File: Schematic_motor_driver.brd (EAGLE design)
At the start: 50 x 50 mm, 29 parts, among them Q2 IRF540, Q3 IRF540, Q4 IRF540, Q5 IRF540, U1 IR2104PBF, U2 IR2104PBF

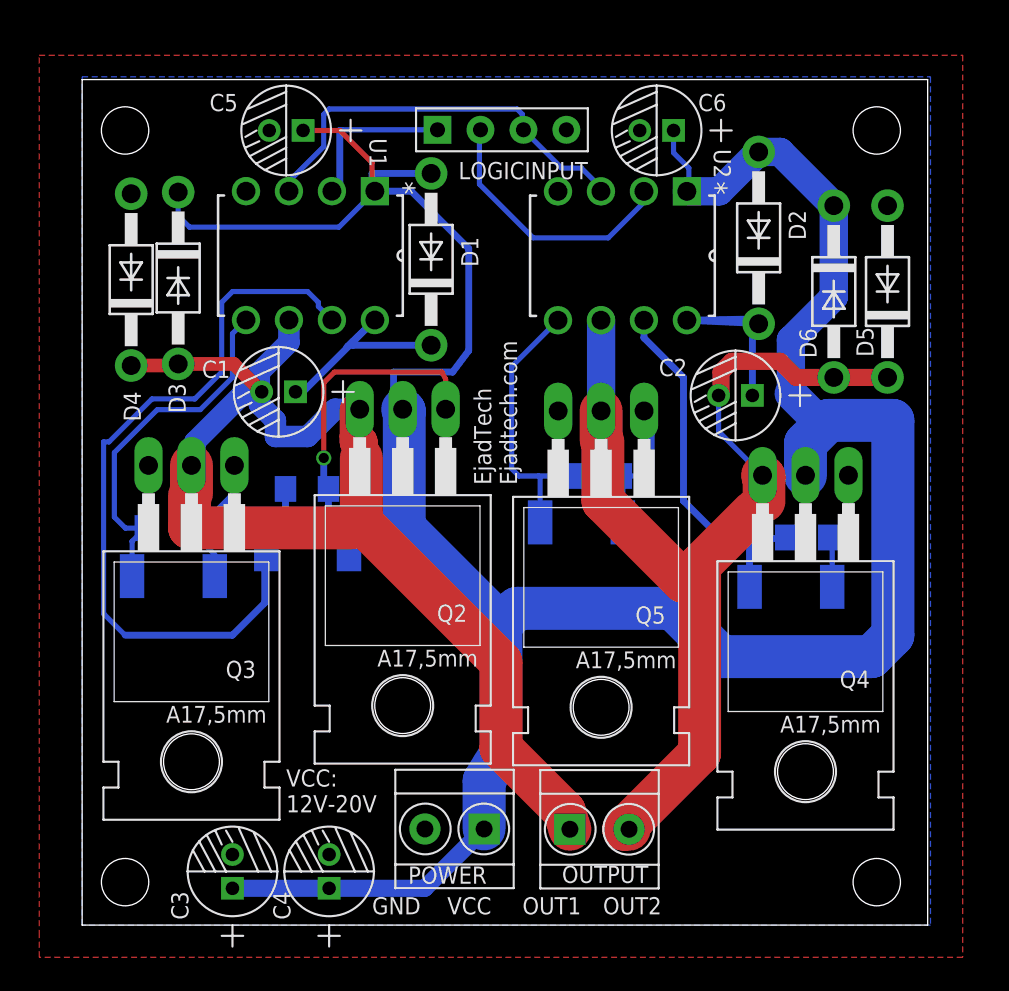
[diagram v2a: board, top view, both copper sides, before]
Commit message: silk adjusted
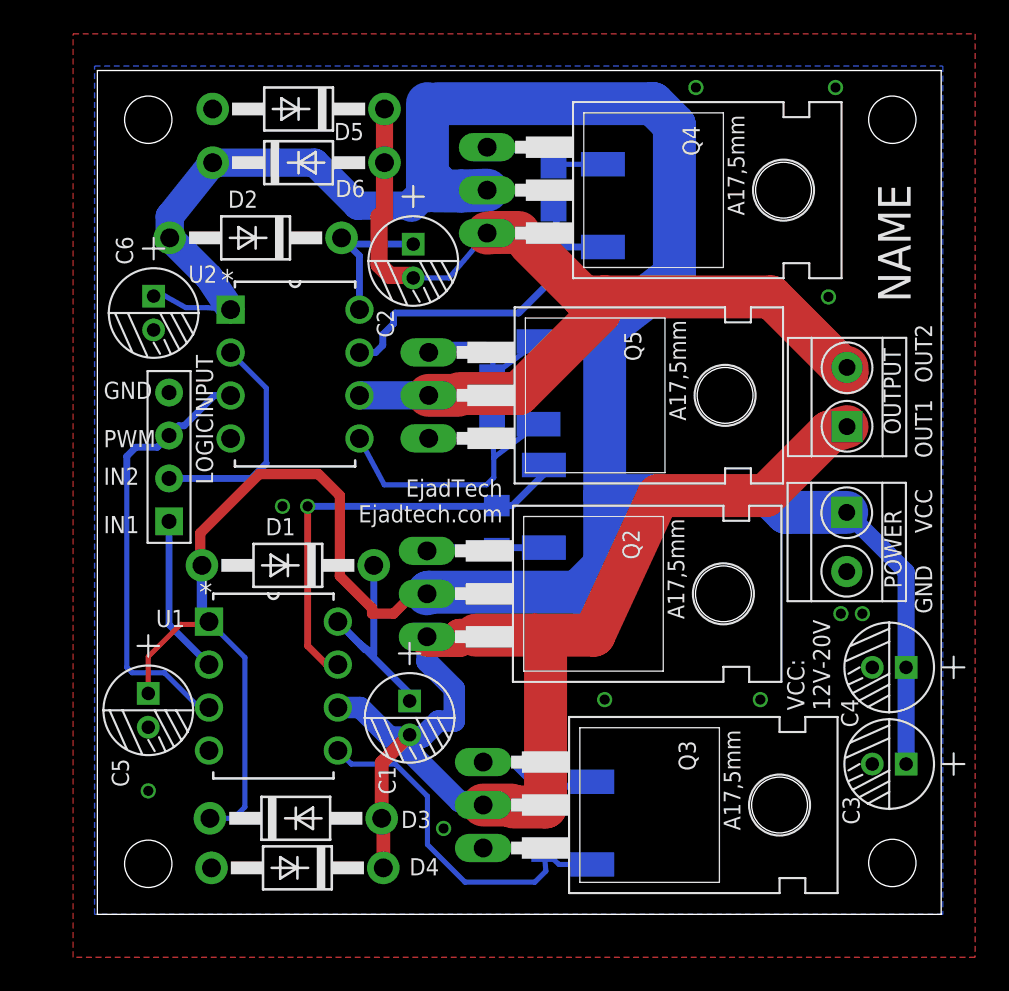
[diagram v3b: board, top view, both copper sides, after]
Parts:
- moved C3 39.4 mm to (47.7, 9.53), turned to 180 degrees
- moved D6 36.5 mm to (12.8, 48.3), turned to 180 degrees
- moved D4 36.1 mm to (12.7, 3.38), turned to 180 degrees
- moved C4 35.2 mm to (47.7, 15.2), turned to 180 degrees
- moved C5 35.2 mm to (3.91, 12.7), turned to 270 degrees
- moved D3 32.7 mm to (12.6, 6.32), turned to 0 degrees
- moved D5 32.6 mm to (12.8, 45.1), turned to 0 degrees
- moved C6 31.6 mm to (4.23, 36.2), turned to 270 degrees
- moved D2 29.7 mm to (10.3, 40.6), turned to 180 degrees
- moved OUTPUT 29.5 mm to (45.2, 31.2), turned to 90 degrees
- moved D8 28.8 mm to (30.2, 6.03), turned to 90 degrees
- moved POWER 28.7 mm to (45.2, 22.7), turned to 270 degrees
- moved R2 28.6 mm to (27.3, 5.64), turned to 90 degrees
- moved LOGICINPUT 27.6 mm to (5.14, 27.7), turned to 180 degrees
- moved Q3 27.3 mm to (30.1, 7.10), turned to 270 degrees
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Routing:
- net N$7: track 48.7 -> 25.8 mm, vias 0 -> 1
- net N$6: track 20.2 -> 6.99 mm, vias 1 -> 0
- net POWER: track 165.4 -> 174.1 mm
- net N$4: track 13.5 -> 9.08 mm
- net IN2: track 16.9 -> 13.6 mm
- net VS1: track 73.8 -> 75.8 mm
- net N$2: track 13.6 -> 15.1 mm
- net VS2: track 61.0 -> 59.8 mm
- net PWM: track 24.7 -> 26.0 mm
- net N$5: track 8.32 -> 8.94 mm
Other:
- board size 50 x 50 mm -> 49.9 x 49.9 mm
- board text added: "IN1"
- board text added: "IN2"
- board text added: "NAME"
- board text added: "PWM"

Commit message: final reviewed. Completed
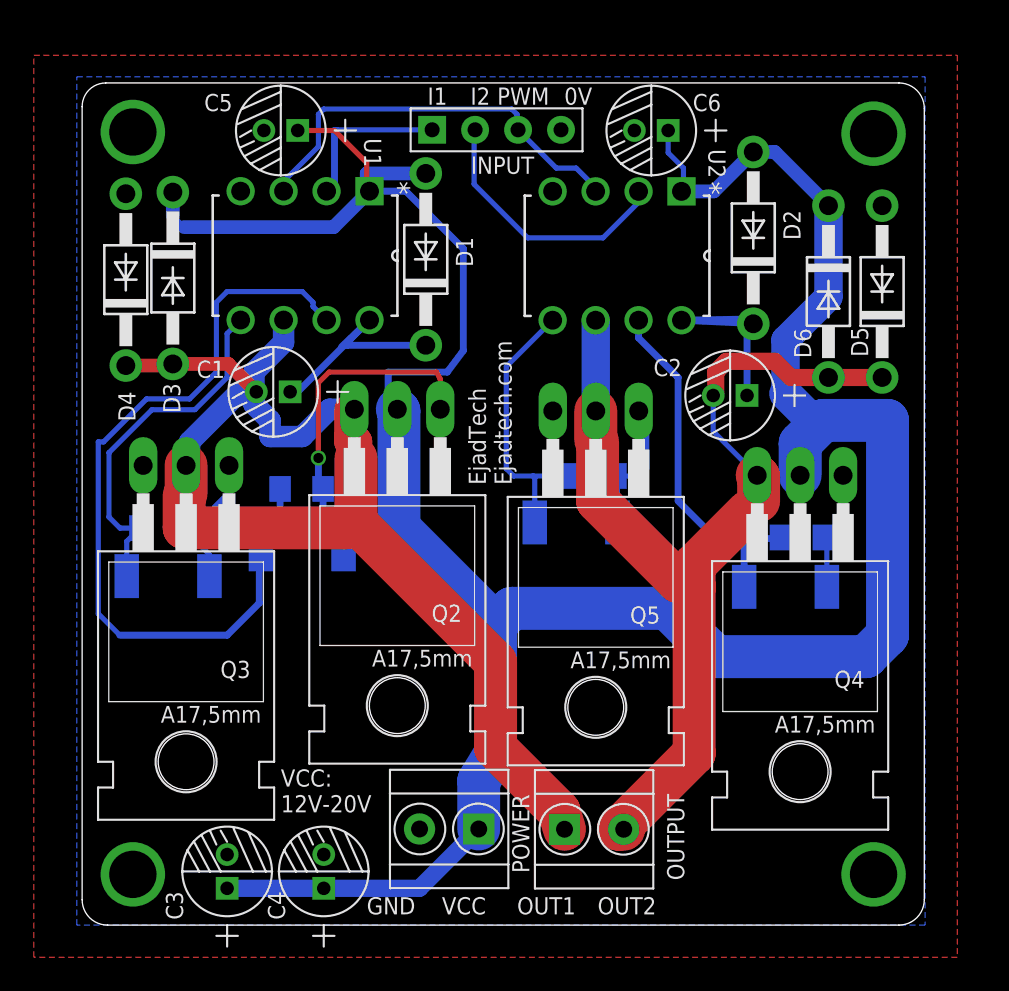
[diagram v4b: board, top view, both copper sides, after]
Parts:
- removed LOGICINPUT: 4p-2.54, Seeed-Connector -2016:H4-2.54
- added INPUT: 4p-2.54, Seeed-Connector -2016:H4-2.54
- moved C3 39.7 mm to (8.57, 3.17), turned to 90 degrees
- moved D4 36.2 mm to (2.58, 38.2), turned to 90 degrees
- moved D6 36.2 mm to (47.3, 37.5), turned to 90 degrees
- moved C4 35.5 mm to (14.3, 3.17), turned to 90 degrees
- moved C5 35.2 mm to (11.7, 47.0), turned to 180 degrees
- moved D3 32.8 mm to (5.36, 38.3), turned to 270 degrees
- moved D5 32.2 mm to (44.1, 37.5), turned to 270 degrees
- moved C6 31.3 mm to (33.7, 47.0), turned to 180 degrees
- moved OUTPUT 29.6 mm to (30.3, 5.67), turned to 0 degrees
- moved D2 29.4 mm to (39.7, 40.6), turned to 90 degrees
- moved D8 29.0 mm to (5.08, 20.6), turned to 180 degrees
- moved POWER 29.0 mm to (21.7, 5.68), turned to 180 degrees
- moved R2 28.8 mm to (4.69, 23.5), turned to 180 degrees
- moved Q3 27.6 mm to (6.15, 20.8), turned to 180 degrees
- moved Q4 26.2 mm to (42.5, 20.2), turned to 180 degrees
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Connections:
- net GND: now also INPUT.4; no longer LOGICINPUT.4
- net IN1: now also INPUT.1; no longer LOGICINPUT.1
- net IN2: now also INPUT.2; no longer LOGICINPUT.2
- net PWM: now also INPUT.3; no longer LOGICINPUT.3
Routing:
- net N$7: track 25.8 -> 48.7 mm, vias 1 -> 0
- net N$6: track 6.99 -> 20.2 mm, vias 0 -> 1
- net POWER: track 174.1 -> 165.4 mm
- net N$4: track 9.08 -> 13.5 mm
- net IN2: track 13.6 -> 16.9 mm
- net VS1: track 75.8 -> 73.8 mm
- net N$2: track 15.1 -> 13.6 mm
- net VS2: track 59.8 -> 61.0 mm
- net PWM: track 26.0 -> 24.7 mm
- net N$5: track 8.94 -> 8.32 mm
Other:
- board size 49.9 x 49.9 mm -> 49.8 x 49.8 mm
- board text added: "0V"
- board text added: "I1"
- board text added: "I2"
- board text added: "Logic Voltage: 3V, 5V and 15V"
- board text removed: "IN1"
- board text removed: "IN2"
- board text removed: "NAME"
